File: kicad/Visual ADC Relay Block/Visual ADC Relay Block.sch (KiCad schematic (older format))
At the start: 21 parts, among them J1 Conn_01x02, J2 Output1, J3 Conn_01x03, J4 Conn_01x02, J5 Output2, K1 DIPxx-1Cxx-51x, Q1 MOSFET_N, Q2 MOSFET_N

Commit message: before changing to ribbons
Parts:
- removed J3: Conn_01x03, Connector_PinSocket_2.54mm:PinSocket_1x03_P2.54mm_Horizontal, symbol Connector_Generic:Conn_01x03
- removed J4: Conn_01x02, Connector_PinSocket_2.54mm:PinSocket_1x02_P2.54mm_Horizontal, symbol Connector_Generic:Conn_01x02
- removed J5: Output2, Connector_PinHeader_2.54mm:PinHeader_1x02_P2.54mm_Horizontal, symbol Connector_Generic:Conn_01x02
- removed Q1, Q2: MOSFET_N, My Libraries:DIP-4_W7.62mm_LongPads_for_IRLD110, symbol My_Library:IRLD110P
- added C1, C2: 1uF, Capacitor_SMD:C_0805_2012Metric_Pad1.18x1.45mm_HandSolder, symbol Device:C_Small
- added J3: Data In, Connector_PinSocket_2.54mm:PinSocket_1x04_P2.54mm_Horizontal, symbol Connector_Generic:Conn_01x04
- added J4: Data Out, Connector_PinHeader_2.54mm:PinHeader_1x04_P2.54mm_Horizontal, symbol Connector_Generic:Conn_01x04
- added J5: PWR In, Connector_PinSocket_2.54mm:PinSocket_1x03_P2.54mm_Horizontal, symbol Connector_Generic:Conn_01x03
- added J6: PWR Out, Connector_PinHeader_2.54mm:PinHeader_1x03_P2.54mm_Horizontal, symbol Connector_Generic:Conn_01x03
- added J? (x2): Conn_02x04_Counter_Clockwise, symbol Connector_Generic:Conn_02x04_Counter_Clockwise
- added Q1: P-NMOS, Package_TO_SOT_SMD:SOT-23, symbol Device:Q_PMOS_GSD
- added R6, R7, R8, R9: R, Resistor_SMD:R_0805_2012Metric_Pad1.20x1.40mm_HandSolder, symbol Device:R_Small
- added U1: 74HCT595, Package_SO:SO-16_3.9x9.9mm_P1.27mm, symbol 74xx:74HCT595
- added U2: 74HC245, Package_SO:SOIC-20W_7.5x12.8mm_P1.27mm, symbol 74xx:74HC245
- J1: value Conn_01x02 -> DAC Vin
- J2: value Output1 -> DAC Vout
- R1, R2: footprint Resistor_THT:R_Axial_DIN0207_L6.3mm_D2.5mm_P7.62mm_Horizontal -> Resistor_SMD:R_0805_2012Metric_Pad1.20x1.40mm_HandSolder
- R3, R4: footprint Resistor_SMD:R_0805_2012Metric_Pad1.15x1.40mm_HandSolder -> Resistor_SMD:R_0805_2012Metric_Pad1.20x1.40mm_HandSolder
- R5: value 2R -> R; footprint Resistor_SMD:R_0805_2012Metric_Pad1.15x1.40mm_HandSolder -> Resistor_SMD:R_0805_2012Metric_Pad1.20x1.40mm_HandSolder
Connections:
- net labels added: CLK, DataIn, DataOut, LATCH, LED1, LED2, LED3, LED4, LED5, LED6, PFET, VCC, VOut
- net labels removed: BitEnable, LEDEnable
- wire segments 64 -> 117
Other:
- note removed: "20 mA * 6 = 120 mA"
- note removed: "5-2 = 3V * 120 mA = 360 mW\n3V/120mA = 25 ohm\n\n5-3.3 = 1.7v * 120 mA = 204 mW\n5/1.7 = 14ohm (120 mA)\n 25ohm (~60 mA)"
- moved on the sheet: D1, JP1, K1, R1, R2, R4

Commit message: time to clean up
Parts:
- removed J1: DAC Vin, Connector_PinSocket_2.54mm:PinSocket_1x02_P2.54mm_Horizontal, symbol Connector_Generic:Conn_01x02
- removed J2: DAC Vout, Connector_PinHeader_2.54mm:PinHeader_1x02_P2.54mm_Horizontal, symbol Connector_Generic:Conn_01x02
- removed J3: Data In, Connector_PinSocket_2.54mm:PinSocket_1x04_P2.54mm_Horizontal, symbol Connector_Generic:Conn_01x04
- removed J4: Data Out, Connector_PinHeader_2.54mm:PinHeader_1x04_P2.54mm_Horizontal, symbol Connector_Generic:Conn_01x04
- removed J5: PWR In, Connector_PinSocket_2.54mm:PinSocket_1x03_P2.54mm_Horizontal, symbol Connector_Generic:Conn_01x03
- removed J6: PWR Out, Connector_PinHeader_2.54mm:PinHeader_1x03_P2.54mm_Horizontal, symbol Connector_Generic:Conn_01x03
- added C? (x4): 22uF, Capacitor_SMD:C_0805_2012Metric_Pad1.18x1.45mm_HandSolder, symbol Device:C_Small
- added JP2: Vref, Jumper:SolderJumper-2_P1.3mm_Open_TrianglePad1.0x1.5mm, symbol Jumper:SolderJumper_2_Open
- J1: renamed from J?; value Conn_02x04_Counter_Clockwise -> In; footprint (none) -> Connector_PinHeader_2.54mm:PinHeader_2x04_P2.54mm_Vertical
- J2: renamed from J?; value Conn_02x04_Counter_Clockwise -> Out; footprint (none) -> Connector_PinHeader_2.54mm:PinHeader_2x04_P2.54mm_Vertical
- JP1: value SolderJumper_2_Open -> First_Module
- R1, R2: footprint Resistor_SMD:R_0805_2012Metric_Pad1.20x1.40mm_HandSolder -> Resistor_THT:R_Axial_DIN0207_L6.3mm_D2.5mm_P10.16mm_Horizontal
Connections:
- wire segments 117 -> 121
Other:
- moved on the sheet: JP1

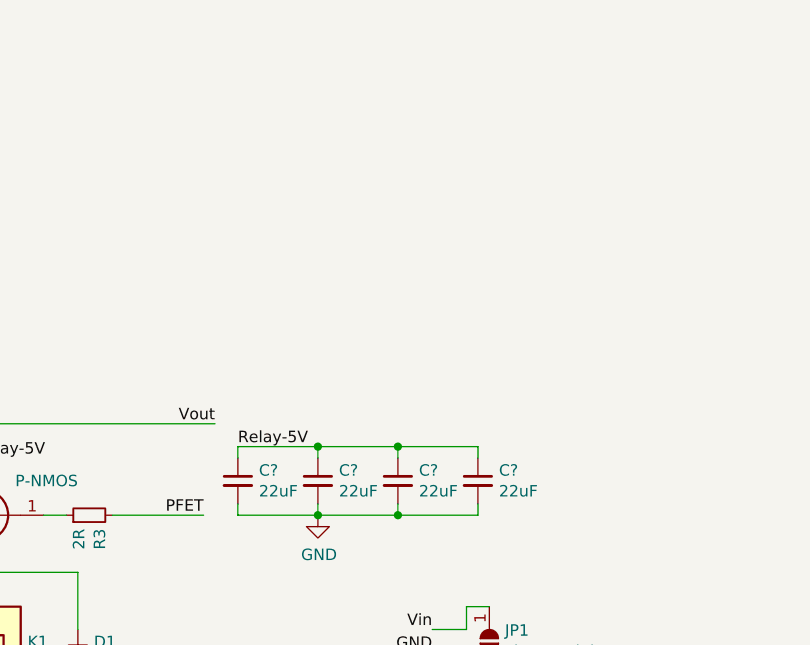
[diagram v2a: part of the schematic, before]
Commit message: why won't you stop
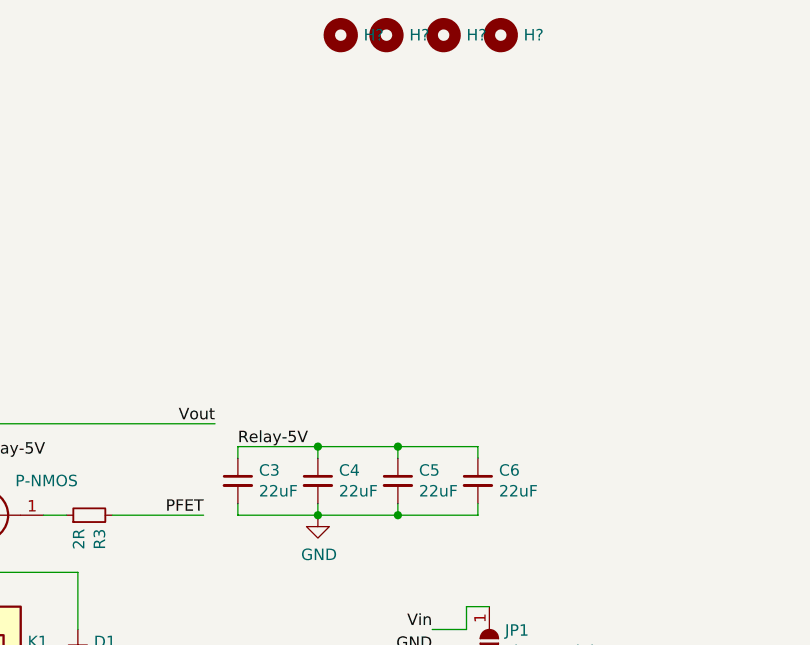
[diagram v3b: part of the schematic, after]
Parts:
- added H? (x4): MountingHole, MountingHole:MountingHole_2.7mm, symbol Mechanical:MountingHole
- gave numbers to parts that had none: 4
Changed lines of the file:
@@
 	12700 5900 12700 5950
 $Comp
-L Device:C_Small C?
+L Device:C_Small C3
 U 1 1 604CF5FA
 P 12700 5800
-F 0 "C?" H 12792 5846 50  0000 L CNN
+F 0 "C3" H 12792 5846 50  0000 L CNN
 F 1 "22uF" H 12792 5755 50  0000 L CNN
 F 2 "Capacitor_SMD:C_0805_2012Metric_Pad1.18x1.45mm_HandSolder" H 12700 5800 50  0001 C CNN
@@
 $EndComp
 $Comp
-L Device:C_Small C?
+L Device:C_Small C4
 U 1 1 604CFC66
 P 13050 5800
-F 0 "C?" H 13142 5846 50  0000 L CNN
+F 0 "C4" H 13142 5846 50  0000 L CNN
 F 1 "22uF" H 13142 5755 50  0000 L CNN
 F 2 "Capacitor_SMD:C_0805_2012Metric_Pad1.18x1.45mm_HandSolder" H 13050 5800 50  0001 C CNN
@@
 $EndComp
 $Comp
-L Device:C_Small C?
+L Device:C_Small C5
 U 1 1 604D0036
 P 13400 5800
-F 0 "C?" H 13492 5846 50  0000 L CNN
+F 0 "C5" H 13492 5846 50  0000 L CNN
 F 1 "22uF" H 13492 5755 50  0000 L CNN
 F 2 "Capacitor_SMD:C_0805_2012Metric_Pad1.18x1.45mm_HandSolder" H 13400 5800 50  0001 C CNN
@@
 $EndComp
 $Comp
-L Device:C_Small C?
+L Device:C_Small C6
 U 1 1 604D02C4
 P 13750 5800
-F 0 "C?" H 13842 5846 50  0000 L CNN
+F 0 "C6" H 13842 5846 50  0000 L CNN
 F 1 "22uF" H 13842 5755 50  0000 L CNN
 F 2 "Capacitor_SMD:C_0805_2012Metric_Pad1.18x1.45mm_HandSolder" H 13750 5800 50  0001 C CNN
@@
 Wire Wire Line
 	13400 5650 13050 5650
+$Comp
+L Mechanical:MountingHole H?
+U 1 1 60553553
+P 13850 3850
+F 0 "H?" H 13950 3850 50  0000 L CNN
+F 1 "MountingHole" H 13950 3805 50  0001 L CNN
+F 2 "MountingHole:MountingHole_2.7mm" H 13850 3850 50  0001 C CNN
+F 3 "~" H 13850 3850 50  0001 C CNN
+	1    13850 3850
+	1    0    0    -1
+$EndComp
+$Comp
+L Mechanical:MountingHole H?
+U 1 1 60553DE2
+P 13600 3850
+F 0 "H?" H 13700 3850 50  0000 L CNN
+F 1 "MountingHole" H 13700 3805 50  0001 L CNN
+F 2 "MountingHole:MountingHole_2.7mm" H 13600 3850 50  0001 C CNN
+F 3 "~" H 13600 3850 50  0001 C CNN
+	1    13600 3850
+	1    0    0    -1
+$EndComp
+$Comp
+L Mechanical:MountingHole H?
+U 1 1 60553F0C
+P 13350 3850
+F 0 "H?" H 13450 3850 50  0000 L CNN
+F 1 "MountingHole" H 13450 3805 50  0001 L CNN
+F 2 "MountingHole:MountingHole_2.7mm" H 13350 3850 50  0001 C CNN
+F 3 "~" H 13350 3850 50  0001 C CNN
+	1    13350 3850
+	1    0    0    -1
+$EndComp
+$Comp
+L Mechanical:MountingHole H?
+U 1 1 6055416A
+P 13150 3850
+F 0 "H?" H 13250 3850 50  0000 L CNN
+F 1 "MountingHole" H 13250 3805 50  0001 L CNN
+F 2 "MountingHole:MountingHole_2.7mm" H 13150 3850 50  0001 C CNN
+F 3 "~" H 13150 3850 50  0001 C CNN
+	1    13150 3850
+	1    0    0    -1
+$EndComp
 $EndSCHEMATC

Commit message: Passed DRC and No Rats
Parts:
- J1: value In -> Out
- J2: value Out -> In
- gave numbers to parts that had none: 4
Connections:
- net labels added: CL1, CL2, CL3, CL4, CL5, CL6
- net labels removed: VOut
- wire segments 121 -> 124
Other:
- moved on the sheet: H1, H2, H3, H4
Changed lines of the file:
@@
 L Device:LED_Small D2
 U 1 1 60277368
-P 14900 9150
-F 0 "D2" V 14946 9080 50  0001 R CNN
-F 1 "LED_Small" V 14855 9080 50  0001 R CNN
-F 2 "LED_SMD:LED_1206_3216Metric_ReverseMount_Hole1.8x2.4mm" V 14900 9150 50  0001 C CNN
-F 3 "~" V 14900 9150 50  0001 C CNN
-	1    14900 9150
+P 14900 9350
+F 0 "D2" V 14946 9280 50  0001 R CNN
+F 1 "LED_Small" V 14855 9280 50  0001 R CNN
+F 2 "LED_SMD:LED_1206_3216Metric_ReverseMount_Hole1.8x2.4mm" V 14900 9350 50  0001 C CNN
+F 3 "~" V 14900 9350 50  0001 C CNN
+	1    14900 9350
 	0    -1   -1   0
 $EndComp
@@
 L Device:LED_Small D3
 U 1 1 60279C79
-P 15050 9150
-F 0 "D3" V 15096 9080 50  0001 R CNN
-F 1 "LED_Small" V 15005 9080 50  0001 R CNN
-F 2 "LED_SMD:LED_1206_3216Metric_ReverseMount_Hole1.8x2.4mm" V 15050 9150 50  0001 C CNN
-F 3 "~" V 15050 9150 50  0001 C CNN
-	1    15050 9150
+P 15050 9350
+F 0 "D3" V 15096 9280 50  0001 R CNN
+F 1 "LED_Small" V 15005 9280 50  0001 R CNN
+F 2 "LED_SMD:LED_1206_3216Metric_ReverseMount_Hole1.8x2.4mm" V 15050 9350 50  0001 C CNN
+F 3 "~" V 15050 9350 50  0001 C CNN
+	1    15050 9350
 	0    -1   -1   0
 $EndComp
@@
 L Device:LED_Small D4
 U 1 1 6027A13B
-P 14750 9150
-F 0 "D4" V 14796 9080 50  0001 R CNN
-F 1 "LED_Small" V 14705 9080 50  0001 R CNN
-F 2 "LED_SMD:LED_1206_3216Metric_ReverseMount_Hole1.8x2.4mm" V 14750 9150 50  0001 C CNN
-F 3 "~" V 14750 9150 50  0001 C CNN
-	1    14750 9150
+P 14750 9350
+F 0 "D4" V 14796 9280 50  0001 R CNN
+F 1 "LED_Small" V 14705 9280 50  0001 R CNN
+F 2 "LED_SMD:LED_1206_3216Metric_ReverseMount_Hole1.8x2.4mm" V 14750 9350 50  0001 C CNN
+F 3 "~" V 14750 9350 50  0001 C CNN
+	1    14750 9350
 	0    -1   -1   0
 $EndComp
@@
 L Device:LED_Small D5
 U 1 1 6027A56C
-P 15500 9150
-F 0 "D5" V 15546 9080 50  0001 R CNN
-F 1 "LED_Small" V 15455 9080 50  0001 R CNN
-F 2 "LED_SMD:LED_1206_3216Metric_ReverseMount_Hole1.8x2.4mm" V 15500 9150 50  0001 C CNN
-F 3 "~" V 15500 9150 50  0001 C CNN
-	1    15500 9150
+P 15500 9350
+F 0 "D5" V 15546 9280 50  0001 R CNN
+F 1 "LED_Small" V 15455 9280 50  0001 R CNN
+F 2 "LED_SMD:LED_1206_3216Metric_ReverseMount_Hole1.8x2.4mm" V 15500 9350 50  0001 C CNN
+F 3 "~" V 15500 9350 50  0001 C CNN
+	1    15500 9350
 	0    -1   -1   0
 $EndComp
@@
 L power:GND #PWR04
 U 1 1 6022E166
-P 15050 9400
-F 0 "#PWR04" H 15050 9150 50  0001 C CNN
-F 1 "GND" H 15055 9227 50  0000 C CNN
-F 2 "" H 15050 9400 50  0001 C CNN
-F 3 "" H 15050 9400 50  0001 C CNN
-	1    15050 9400
+P 15050 9600
+F 0 "#PWR04" H 15050 9350 50  0001 C CNN
+F 1 "GND" H 15055 9427 50  0000 C CNN
+F 2 "" H 15050 9600 50  0001 C CNN
+F 3 "" H 15050 9600 50  0001 C CNN
+	1    15050 9600
 	1    0    0    -1
 $EndComp
@@
 L Device:LED_Small D6
 U 1 1 60259EEF
-P 15200 9150
-F 0 "D6" V 15246 9080 50  0001 R CNN
-F 1 "LED_Small" V 15155 9080 50  0001 R CNN
-F 2 "LED_SMD:LED_1206_3216Metric_ReverseMount_Hole1.8x2.4mm" V 15200 9150 50  0001 C CNN
-F 3 "~" V 15200 9150 50  0001 C CNN
-	1    15200 9150
+P 15200 9350
+F 0 "D6" V 15246 9280 50  0001 R CNN
+F 1 "LED_Small" V 15155 9280 50  0001 R CNN
+F 2 "LED_SMD:LED_1206_3216Metric_ReverseMount_Hole1.8x2.4mm" V 15200 9350 50  0001 C CNN
+F 3 "~" V 15200 9350 50  0001 C CNN
+	1    15200 9350
 	0    -1   -1   0
 $EndComp
@@
 L Device:LED_Small D7
 U 1 1 60259EF5
-P 15350 9150
-F 0 "D7" V 15396 9080 50  0001 R CNN
-F 1 "LED_Small" V 15305 9080 50  0001 R CNN
-F 2 "LED_SMD:LED_1206_3216Metric_ReverseMount_Hole1.8x2.4mm" V 15350 9150 50  0001 C CNN
-F 3 "~" V 15350 9150 50  0001 C CNN
-	1    15350 9150
+P 15350 9350
+F 0 "D7" V 15396 9280 50  0001 R CNN
+F 1 "LED_Small" V 15305 9280 50  0001 R CNN
+F 2 "LED_SMD:LED_1206_3216Metric_ReverseMount_Hole1.8x2.4mm" V 15350 9350 50  0001 C CNN
+F 3 "~" V 15350 9350 50  0001 C CNN
+	1    15350 9350
 	0    -1   -1   0
 $EndComp
 Wire Wire Line
-	14750 9250 14750 9300
-Wire Wire Line
-	15500 9300 15500 9250
-Wire Wire Line
-	15350 9250 15350 9300
-Connection ~ 15350 9300
-Wire Wire Line
-	15350 9300 15500 9300
-Wire Wire Line
-	15200 9250 15200 9300
-Wire Wire Line
-	14750 9300 14900 9300
-Connection ~ 15200 9300
-Wire Wire Line
-	15200 9300 15350 9300
-Wire Wire Line
-	15050 9250 15050 9300
-Connection ~ 15050 9300
-Wire Wire Line
-	15050 9300 15200 9300
-Wire Wire Line
-	14900 9250 14900 9300
-Connection ~ 14900 9300
-Wire Wire Line
-	14900 9300 15050 9300
-Wire Wire Line
-	14750 9050 14750 8850
-Wire Wire Line
-	15350 8850 15350 9050
-Wire Wire Line
-	15050 9050 15050 8850
-Wire Wire Line
-	15050 9300 15050 9400
+	14750 9450 14750 9500
+Wire Wire Line
+	15500 9500 15500 9450
+Wire Wire Line
+	15350 9450 15350 9500
+Connection ~ 15350 9500
+Wire Wire Line
+	15350 9500 15500 9500
+Wire Wire Line
+	15200 9450 15200 9500
+Wire Wire Line
+	14750 9500 14900 9500
+Connection ~ 15200 9500
+Wire Wire Line
+	15200 9500 15350 9500
+Wire Wire Line
+	15050 9450 15050 9500
+Connection ~ 15050 9500
+Wire Wire Line
+	15050 9500 15200 9500
+Wire Wire Line
+	14900 9450 14900 9500
+Connection ~ 14900 9500
+Wire Wire Line
+	14900 9500 15050 9500
+Wire Wire Line
+	15050 9500 15050 9600
 Wire Wire Line
 	10800 5550 11150 5550
@@
 Wire Wire Line
 	15500 8850 15500 8400
+Text Label 15050 8400 3    50   ~ 0
+LED1
 Text Label 14750 8400 3    50   ~ 0
-LED1
-Text Label 14900 8400 3    50   ~ 0
 LED2
-Text Label 15050 8400 3    50   ~ 0
+Text Label 15500 8400 3    50   ~ 0
 LED3
 Text Label 15200 8400 3    50   ~ 0
@@
 Text Label 15350 8400 3    50   ~ 0
 LED5
-Text Label 15500 8400 3    50   ~ 0
+Text Label 14900 8400 3    50   ~ 0
 LED6
 Wire Wire Line
@@
 P 9600 6950
 F 0 "J2" H 9650 7267 50  0000 C CNN
-F 1 "Out" H 9650 7176 50  0000 C CNN
+F 1 "In" H 9650 7176 50  0000 C CNN
 F 2 "Connector_PinHeader_2.54mm:PinHeader_2x04_P2.54mm_Vertical" H 9600 6950 50  0001 C CNN
 F 3 "~" H 9600 6950 50  0001 C CNN
@@
 P 9600 6200
 F 0 "J1" H 9650 6517 50  0000 C CNN
-F 1 "In" H 9650 6426 50  0000 C CNN
+F 1 "Out" H 9650 6426 50  0000 C CNN
 F 2 "Connector_PinHeader_2.54mm:PinHeader_2x04_P2.54mm_Vertical" H 9600 6200 50  0001 C CNN
 F 3 "~" H 9600 6200 50  0001 C CNN
@@
 	9400 6400 9050 6400
 Text Label 10300 6300 2    50   ~ 0
-VOut
+Vout
 Wire Wire Line
 	10300 6300 9900 6300
@@
 	13400 5650 13050 5650
 $Comp
-L Mechanical:MountingHole H?
+L Mechanical:MountingHole H4
 U 1 1 60553553
-P 13850 3850
-F 0 "H?" H 13950 3850 50  0000 L CNN
-F 1 "MountingHole" H 13950 3805 50  0001 L CNN
-F 2 "MountingHole:MountingHole_2.7mm" H 13850 3850 50  0001 C CNN
-F 3 "~" H 13850 3850 50  0001 C CNN
-	1    13850 3850
-	1    0    0    -1
-$EndComp
-$Comp
-L Mechanical:MountingHole H?
+P 13600 4550
+F 0 "H4" H 13700 4550 50  0000 L CNN
+F 1 "MountingHole" H 13700 4505 50  0001 L CNN
+F 2 "MountingHole:MountingHole_2.7mm" H 13600 4550 50  0001 C CNN
+F 3 "~" H 13600 4550 50  0001 C CNN
+	1    13600 4550
+	1    0    0    -1
+$EndComp
+$Comp
+L Mechanical:MountingHole H3
 U 1 1 60553DE2
-P 13600 3850
-F 0 "H?" H 13700 3850 50  0000 L CNN
-F 1 "MountingHole" H 13700 3805 50  0001 L CNN
-F 2 "MountingHole:MountingHole_2.7mm" H 13600 3850 50  0001 C CNN
-F 3 "~" H 13600 3850 50  0001 C CNN
-	1    13600 3850
-	1    0    0    -1
-$EndComp
-$Comp
-L Mechanical:MountingHole H?
+P 13350 4550
+F 0 "H3" H 13450 4550 50  0000 L CNN
+F 1 "MountingHole" H 13450 4505 50  0001 L CNN
+F 2 "MountingHole:MountingHole_2.7mm" H 13350 4550 50  0001 C CNN
+F 3 "~" H 13350 4550 50  0001 C CNN
+	1    13350 4550
+	1    0    0    -1
+$EndComp
+$Comp
+L Mechanical:MountingHole H2
 U 1 1 60553F0C
-P 13350 3850
-F 0 "H?" H 13450 3850 50  0000 L CNN
-F 1 "MountingHole" H 13450 3805 50  0001 L CNN
-F 2 "MountingHole:MountingHole_2.7mm" H 13350 3850 50  0001 C CNN
-F 3 "~" H 13350 3850 50  0001 C CNN
-	1    13350 3850
-	1    0    0    -1
-$EndComp
-$Comp
-L Mechanical:MountingHole H?
+P 13100 4550
+F 0 "H2" H 13200 4550 50  0000 L CNN
+F 1 "MountingHole" H 13200 4505 50  0001 L CNN
+F 2 "MountingHole:MountingHole_2.7mm" H 13100 4550 50  0001 C CNN
+F 3 "~" H 13100 4550 50  0001 C CNN
+	1    13100 4550
+	1    0    0    -1
+$EndComp
+$Comp
+L Mechanical:MountingHole H1
 U 1 1 6055416A
-P 13150 3850
-F 0 "H?" H 13250 3850 50  0000 L CNN
-F 1 "MountingHole" H 13250 3805 50  0001 L CNN
-F 2 "MountingHole:MountingHole_2.7mm" H 13150 3850 50  0001 C CNN
-F 3 "~" H 13150 3850 50  0001 C CNN
-	1    13150 3850
-	1    0    0    -1
-$EndComp
+P 12900 4550
+F 0 "H1" H 13000 4550 50  0000 L CNN
+F 1 "MountingHole" H 13000 4505 50  0001 L CNN
+F 2 "MountingHole:MountingHole_2.7mm" H 12900 4550 50  0001 C CNN
+F 3 "~" H 12900 4550 50  0001 C CNN
+	1    12900 4550
+	1    0    0    -1
+$EndComp
+Wire Wire Line
+	14750 8850 14750 9250
+Wire Wire Line
+	14900 9050 14900 9250
+Wire Wire Line
+	15050 8850 15050 9250
+Wire Wire Line
+	15200 9050 15200 9250
+Wire Wire Line
+	15500 9050 15500 9250
+Wire Wire Line
+	15350 8850 15350 9250
+Text Label 15050 9100 3    50   ~ 0
+CL1
+Text Label 14750 9100 3    50   ~ 0
+CL2
+Text Label 15500 9100 3    50   ~ 0
+CL3
+Text Label 15350 9100 3    50   ~ 0
+CL5
+Text Label 14900 9100 3    50   ~ 0
+CL6
+Text Label 15200 9100 3    50   ~ 0
+CL4
 $EndSCHEMATC

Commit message: change in/out but need to save brains
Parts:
- J1, J2: symbol Connector_Generic:Conn_02x04_Counter_Clockwise -> Connector_Generic:Conn_02x04_Odd_Even
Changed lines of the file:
@@
 Text Label 14900 8400 3    50   ~ 0
 LED6
-Wire Wire Line
-	9400 7050 9050 7050
-Text Label 9050 7050 0    50   ~ 0
-DataIn
-Wire Wire Line
-	9400 6950 9050 6950
-Text Label 9050 6950 0    50   ~ 0
+$Comp
+L Connector_Generic:Conn_02x04_Odd_Even J2
+U 1 1 603C4B3A
+P 8350 6850
+F 0 "J2" H 8400 7167 50  0000 C CNN
+F 1 "In" H 8400 7076 50  0000 C CNN
+F 2 "Connector_PinHeader_2.54mm:PinHeader_2x04_P2.54mm_Vertical" H 8350 6850 50  0001 C CNN
+F 3 "~" H 8350 6850 50  0001 C CNN
+	1    8350 6850
+	1    0    0    -1
+$EndComp
+Wire Wire Line
+	6600 6850 6200 6850
+Text Label 6200 6850 0    50   ~ 0
+DataOut
+Wire Wire Line
+	7100 6750 7500 6750
+Text Label 7500 6750 2    50   ~ 0
 CLK
 Wire Wire Line
-	9400 6850 9050 6850
-Text Label 9050 6850 0    50   ~ 0
+	6600 6750 6200 6750
+Text Label 6200 6750 0    50   ~ 0
 LATCH
-Text Label 10300 6850 2    50   ~ 0
+Text Label 7500 7050 2    50   ~ 0
 Relay-5V
-Text Label 10300 6950 2    50   ~ 0
+Text Label 6200 7050 0    50   ~ 0
 Vref
-Text Label 10300 7150 2    50   ~ 0
-GND
-$Comp
-L Connector_Generic:Conn_02x04_Counter_Clockwise J2
-U 1 1 603C4B3A
-P 9600 6950
-F 0 "J2" H 9650 7267 50  0000 C CNN
-F 1 "In" H 9650 7176 50  0000 C CNN
-F 2 "Connector_PinHeader_2.54mm:PinHeader_2x04_P2.54mm_Vertical" H 9600 6950 50  0001 C CNN
-F 3 "~" H 9600 6950 50  0001 C CNN
-	1    9600 6950
-	1    0    0    -1
-$EndComp
-Wire Wire Line
-	9400 7150 9050 7150
-Text Label 10300 7050 2    50   ~ 0
-Vin
-Wire Wire Line
-	10300 7050 9900 7050
-Wire Wire Line
-	10300 6950 9900 6950
-Wire Wire Line
-	10300 7150 9900 7150
-Wire Wire Line
-	9900 6850 10300 6850
-Text Label 9050 7150 0    50   ~ 0
-GND
-Wire Wire Line
-	9400 6300 9050 6300
-Text Label 9050 6300 0    50   ~ 0
-DataOut
-Wire Wire Line
-	9400 6200 9050 6200
-Text Label 9050 6200 0    50   ~ 0
-CLK
-Wire Wire Line
-	9400 6100 9050 6100
-Text Label 9050 6100 0    50   ~ 0
-LATCH
-Text Label 10300 6100 2    50   ~ 0
-Relay-5V
-Text Label 10300 6200 2    50   ~ 0
-Vref
-Text Label 10300 6400 2    50   ~ 0
-GND
-$Comp
-L Connector_Generic:Conn_02x04_Counter_Clockwise J1
+$Comp
+L Connector_Generic:Conn_02x04_Odd_Even J1
 U 1 1 603E750E
-P 9600 6200
-F 0 "J1" H 9650 6517 50  0000 C CNN
-F 1 "Out" H 9650 6426 50  0000 C CNN
-F 2 "Connector_PinHeader_2.54mm:PinHeader_2x04_P2.54mm_Vertical" H 9600 6200 50  0001 C CNN
-F 3 "~" H 9600 6200 50  0001 C CNN
-	1    9600 6200
-	1    0    0    -1
-$EndComp
-Wire Wire Line
-	9400 6400 9050 6400
-Text Label 10300 6300 2    50   ~ 0
-Vout
-Wire Wire Line
-	10300 6300 9900 6300
-Wire Wire Line
-	10300 6200 9900 6200
-Wire Wire Line
-	10300 6400 9900 6400
-Wire Wire Line
-	9900 6100 10300 6100
-Text Label 9050 6400 0    50   ~ 0
+P 6800 6850
+F 0 "J1" H 6850 7167 50  0000 C CNN
+F 1 "Out" H 6850 7076 50  0000 C CNN
+F 2 "Connector_PinHeader_2.54mm:PinHeader_2x04_P2.54mm_Vertical" H 6800 6850 50  0001 C CNN
+F 3 "~" H 6800 6850 50  0001 C CNN
+	1    6800 6850
+	1    0    0    -1
+$EndComp
+Wire Wire Line
+	7100 6850 7500 6850
+Wire Wire Line
+	7500 6950 7100 6950
+Wire Wire Line
+	6200 7050 6600 7050
+Wire Wire Line
+	6200 6950 6600 6950
+Wire Wire Line
+	7100 7050 7500 7050
+Text Label 7500 6850 2    50   ~ 0
 GND
 Wire Wire Line
@@
 Text Label 15200 9100 3    50   ~ 0
 CL4
+Wire Wire Line
+	8150 7050 7750 7050
+Wire Wire Line
+	7750 6850 8150 6850
+Wire Wire Line
+	9050 7050 8650 7050
+Wire Wire Line
+	7750 6950 8150 6950
+Text Label 9050 7050 2    50   ~ 0
+Vref
+Text Label 7750 7050 0    50   ~ 0
+Relay-5V
+Text Label 9050 6950 2    50   ~ 0
+GND
+Wire Wire Line
+	8650 6950 9050 6950
+Text Label 9050 6750 2    50   ~ 0
+LATCH
+Wire Wire Line
+	8650 6750 9050 6750
+Text Label 7750 6750 0    50   ~ 0
+CLK
+Wire Wire Line
+	8150 6750 7750 6750
+Text Label 9050 6850 2    50   ~ 0
+DataIn
+Wire Wire Line
+	8650 6850 9050 6850
+Text Label 6200 6950 0    50   ~ 0
+GND
+Text Label 7750 6850 0    50   ~ 0
+GND
+Text Label 7500 6950 2    50   ~ 0
+Vout
+Text Label 7750 6950 0    50   ~ 0
+Vin
 $EndSCHEMATC
